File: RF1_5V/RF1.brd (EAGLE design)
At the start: 7 x 7.1 mm, 13 parts, among them J1 5v, Q1 16mhz, U1 ATMEGA328P_PDIP

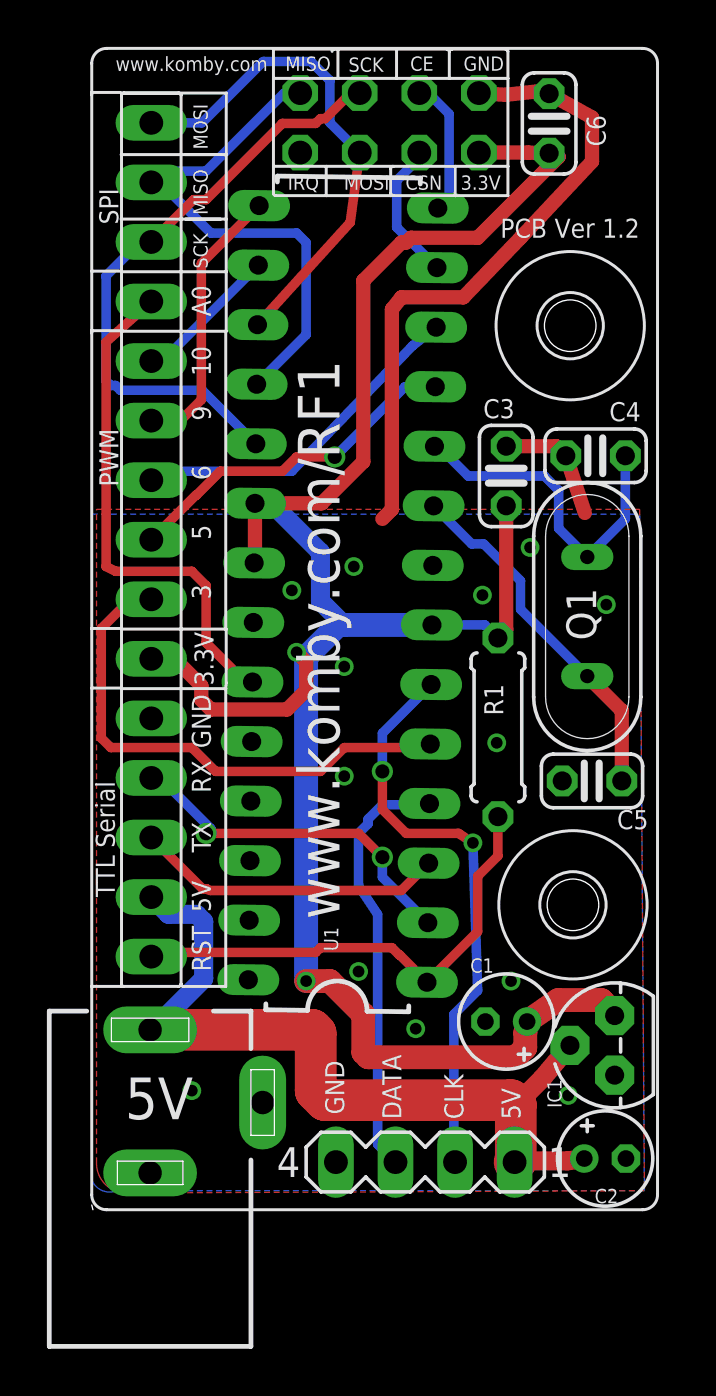
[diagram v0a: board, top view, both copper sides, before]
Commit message: Updated with 2014 designs for both RF1_12v and RF1 5v
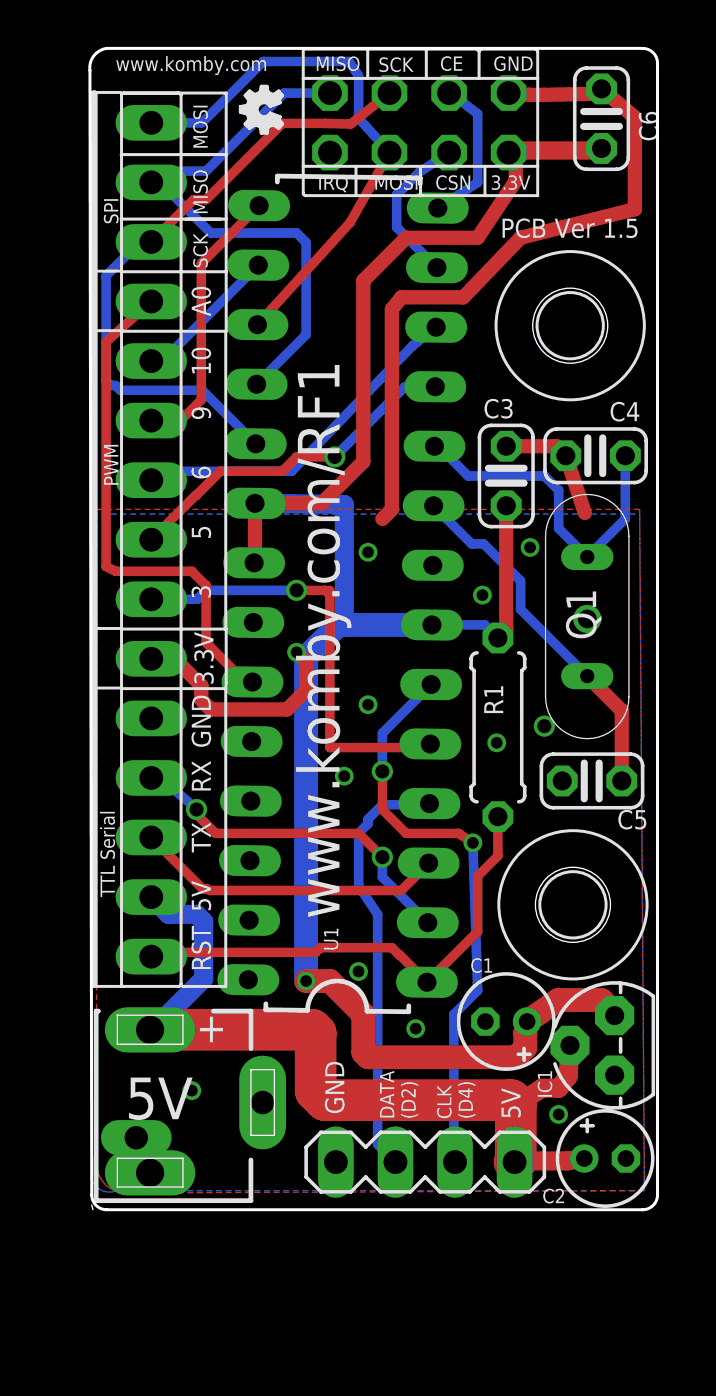
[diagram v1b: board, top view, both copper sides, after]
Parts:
- added U$1: (no value), ohw-logo:OSHW_FILLX70_NOTEXT
- J1: device con-jack:DCJ0303 -> con-jack_komby:DCJ0303
- moved C6 2.24 mm to (21.7, 46.5)
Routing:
- net +3V3: track 93.4 -> 98.8 mm
- net PWM1_D3: track 22.4 -> 18.9 mm, vias 0 -> 1
- net GND: track 32.8 -> 36.1 mm, vias 13 -> 12
- net MOSI: track 21.5 -> 23.3 mm
- net MISO: track 22.5 -> 23.8 mm
- net SCK: track 26.0 -> 27.2 mm
- net RF_CSN: track 6.02 -> 6.70 mm
- net RF_CE: track 5.85 -> 6.46 mm
- net +5V: track 35.5 -> 36.0 mm
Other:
- board size 7 x 7.1 mm -> 24.2 x 49.5 mm
- board text added: "CLK (D4)"
- board text added: "DATA (D2)"
- board text added: "PCB Ver 1.5"
- board text removed: "CLK"
- board text removed: "DATA"
- board text removed: "PCB Ver 1.2"
